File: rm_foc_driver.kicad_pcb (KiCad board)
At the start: 4 copper layers, 70 x 70 mm, 88 parts, among them J1 SWD, J2 TMC4671, J3 UART, J4 TMC4671, J5 Conn_01x03, J6 Conn_01x02, J8 Conn_01x03, Q1 CSD18540Q5B, Q2 CSD18540Q5B, Q3 CSD18540Q5B, Q4 CSD18540Q5B, Q5 CSD18540Q5B, Q6 CSD18540Q5B, U1 TPS54540, U10 74HC244, U2 RT9013, U3 STM32F401CCUx, U4 SY8303, U5 IR2104, U6 INA2180, U7 MT6701, U8 IR2104, U9 IR2104, Y1 Crystal_GND24

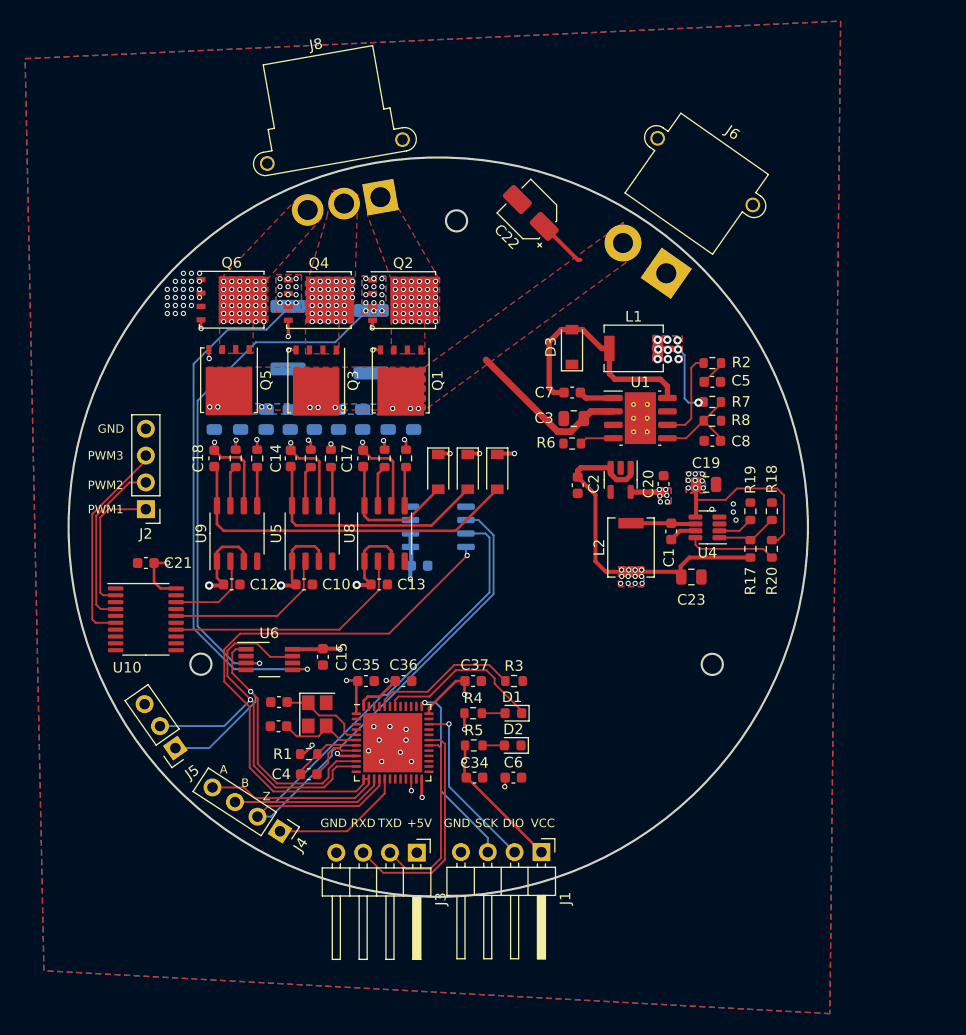
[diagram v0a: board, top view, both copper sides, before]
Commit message: version 1.0.0-beta
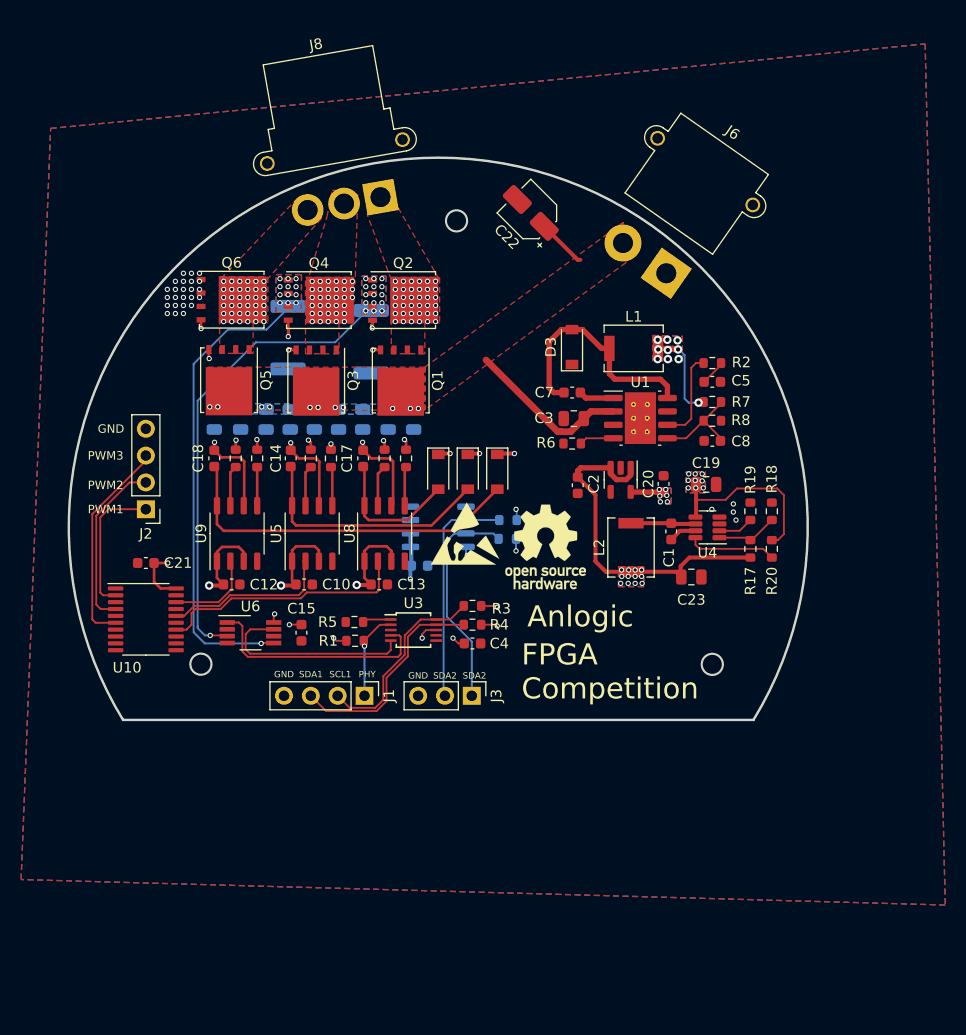
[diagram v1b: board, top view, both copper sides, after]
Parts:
- removed C11, C9: 22pF, Capacitor_SMD:C_0603_1608Metric
- removed C34, C35, C36, C37: 100nF, Capacitor_SMD:C_0603_1608Metric
- removed C6: 4.7uF, Capacitor_SMD:C_0603_1608Metric
- removed D1, D2: LED, LED_SMD:LED_0603_1608Metric
- removed J4: TMC4671, Connector_PinHeader_2.54mm:PinHeader_1x04_P2.54mm_Vertical
- removed J5: Conn_01x03, Connector_PinSocket_2.54mm:PinSocket_1x03_P2.54mm_Vertical
- removed Y1: Crystal_GND24, Crystal:Crystal_SMD_3225-4Pin_3.2x2.5mm
- added R21: 10k, Resistor_SMD:R_0603_1608Metric, B.Cu at (171.7, 100.3)
- added R22: 10k, Resistor_SMD:R_0603_1608Metric, B.Cu at (171.6, 102.1)
- added REF**: ESD-Logo_6.6x6mm_SilkScreen, Symbol:ESD-Logo_6.6x6mm_SilkScreen, F.Cu at (167.6, 101.6)
- added REF**: OSHW-Logo_7.5x8mm_SilkScreen, Symbol:OSHW-Logo_7.5x8mm_SilkScreen, F.Cu at (175.3, 102.9)
- C4: value 100nF -> 1uF
- J1: value SWD -> TMC4671; footprint Connector_PinHeader_2.54mm:PinHeader_1x04_P2.54mm_Horizontal -> Connector_PinHeader_2.54mm:PinHeader_1x04_P2.54mm_Vertical
- J3: value UART -> Conn_01x03; footprint Connector_PinHeader_2.54mm:PinHeader_1x04_P2.54mm_Horizontal -> Connector_PinHeader_2.54mm:PinHeader_1x03_P2.54mm_Vertical
- U3: value STM32F401CCUx -> ADS1115IDGS; footprint Package_DFN_QFN:QFN-48-1EP_7x7mm_P0.5mm_EP5.6x5.6mm -> Package_SO:TSSOP-10_3x3mm_P0.5mm
- moved J1 22.4 mm to (158.1, 117.0)
- moved C4 19.8 mm to (168.3, 112.0)
- moved R5 16.3 mm to (157.2, 110.0)
- moved J3 15.7 mm to (168.3, 117.0)
- moved R1 11.6 mm to (157.2, 111.8), turned to 0 degrees
- moved U3 10.8 mm to (162.8, 110.7)
- moved R4 8.38 mm to (168.3, 110.2), turned to 180 degrees
- moved R3 8.13 mm to (168.3, 108.5), turned to 180 degrees
- moved U6 3.10 mm to (147.3, 111.0)
- moved C15 3.06 mm to (152.1, 111.0)
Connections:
- C4 pad 1: Net-(C4-Pad1) -> +5V
- J1 pad 1: +3.3V -> /RDY
- J1 pad 2: /SWDIO -> /SCL1
- J1 pad 3: /SWCLK -> /SDA1
- J3 pad 1: +5V -> /SCL2
- J3 pad 2: /TXD -> /SDA2
- J3 pad 3: /RXD -> GND
- R1 pad 1: Net-(C4-Pad1) -> +5V
- R1 pad 2: +3.3V -> /RDY
- R3 pad 1: Net-(R3-Pad1) -> +5V
- R3 pad 2: GND -> /SCL1
- R4 pad 1: +3.3V -> +5V
- R4 pad 2: Net-(D1-Pad2) -> /SDA1
- R5 pad 1: +3.3V -> GND
- R5 pad 2: Net-(D2-Pad2) -> Net-(R5-Pad2)
- U3 pad 1: +3.3V -> Net-(R5-Pad2)
- U3 pad 10: /SO1 -> /SCL1
- U3 pad 2: unconnected-(U3-Pad2) -> /RDY
- U3 pad 3: unconnected-(U3-Pad3) -> GND
- U3 pad 4: unconnected-(U3-Pad4) -> /SO1
- U3 pad 5: /OSC_IN -> /SO2
- U3 pad 6: /OSC_OUT -> unconnected-(U3-Pad6)
- U3 pad 7: Net-(C4-Pad1) -> unconnected-(U3-Pad7)
- U3 pad 8: GND -> +5V
- U3 pad 9: +3.3V -> /SDA1
- U7 pad 6: /MISO -> /SDA2
- U7 pad 7: /SCLK -> /SCL2
- U7 pad 8: /CS1 -> +5V
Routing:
- net +3.3V: track 106.9 -> 6.38 mm, vias 14 -> 6
- net /CS1: track 69.0 -> 0.00 mm, vias 1 -> 0
- net /SCLK: track 54.3 -> 0.00 mm
- net /MISO: track 53.5 -> 0.00 mm
- net /RXD: track 21.7 -> 0.00 mm
- net /SDA2: track 0.00 -> 21.5 mm
- net /SO2: track 40.4 -> 19.2 mm, vias 1 -> 0
- net /SCL2: track 0.00 -> 21.0 mm
- net /SDA1: track 0.00 -> 20.8 mm
- net /SCL1: track 0.00 -> 18.8 mm
- net /SWCLK: track 17.7 -> 0.00 mm, vias 1 -> 0
- net /TXD: track 17.5 -> 0.00 mm
- net /SWDIO: track 16.6 -> 0.00 mm, vias 1 -> 0
- net Net-(D1-Pad1): track 15.9 -> 0.00 mm
- net Net-(R3-Pad1): track 14.1 -> 0.00 mm
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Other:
- board size 70 x 70 mm -> 70 x 53.2 mm
- board text added: "Anlogic"
- board text added: "FPGA Competition"
- board text added: "PHY"
- board text added: "SCL1"
- board text added: "SDA1"
- board text added: "SDA2"
- board text removed: "+5V"
- board text removed: "A"
- board text removed: "B"
- board text removed: "DIO"
- board text removed: "RXD"
- board text removed: "SCK"
- board text removed: "TXD"
- board text removed: "VCC"
- board text removed: "Z"
